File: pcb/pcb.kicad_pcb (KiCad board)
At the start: 2 copper layers, 100 x 88.7 mm, 65 parts, among them J1 AudioJack4, J2 USB_C_Receptacle_USB2.0, SW1 Switch, SW10 Switch, SW11 Switch, SW12 Switch, SW13 Switch, SW14 Switch, SW15 Switch, SW16 Switch, SW17 Switch, SW18 Switch, SW2 Switch, SW3 Switch, SW4 Switch, SW5 Switch, SW6 Switch, SW7 Switch, SW8 Switch, SW9 Switch, U1 MCU_rp2040-zero, U2 MCU_rp2040-zero, U3 RollerEncoder_EVQWGD001

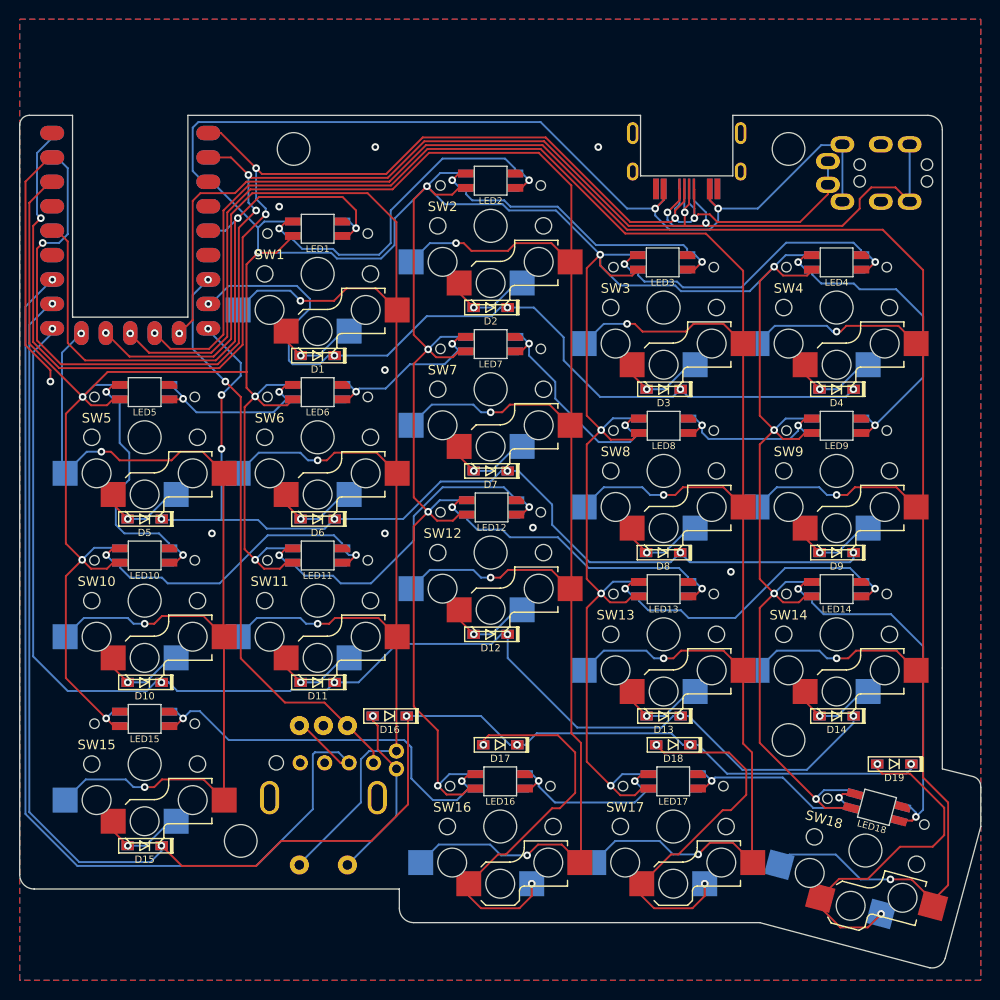
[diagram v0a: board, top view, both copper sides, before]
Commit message: small PCB updates
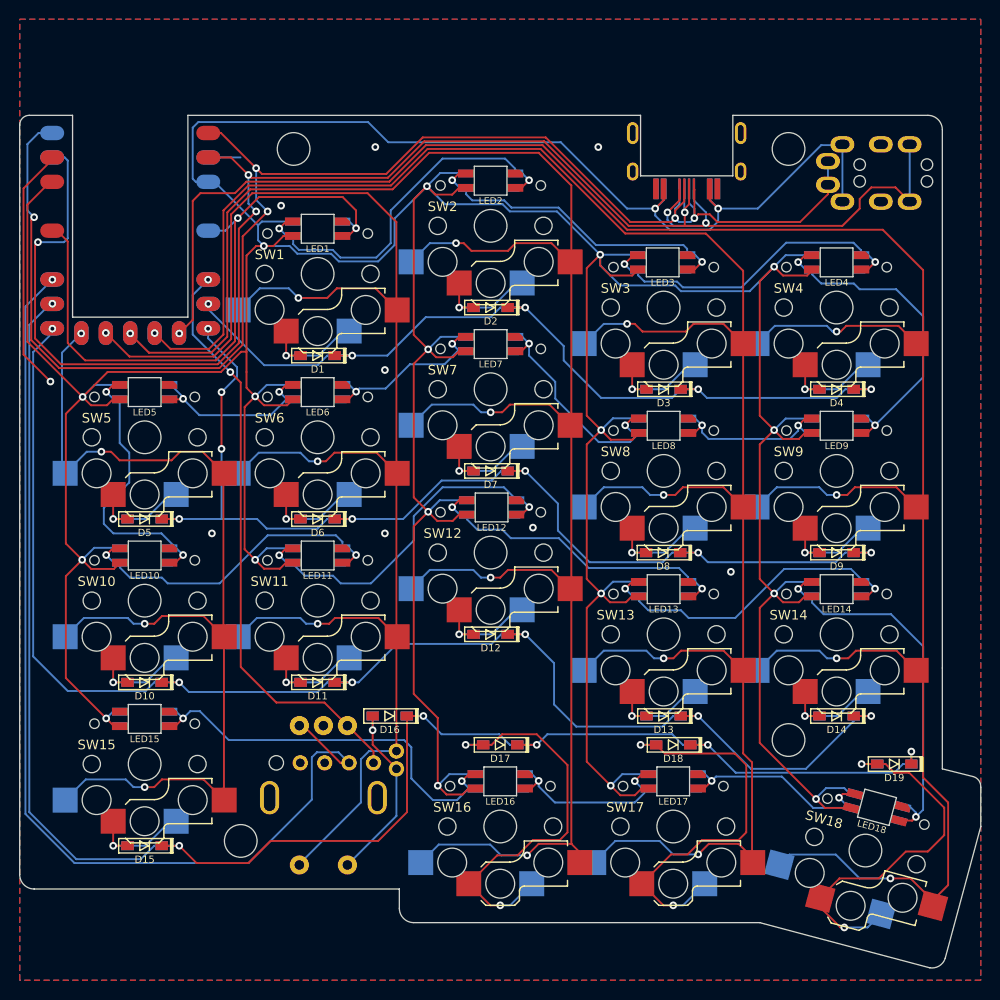
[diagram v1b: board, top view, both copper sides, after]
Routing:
- net row2: track 136.0 -> 149.7 mm
- net row1: track 103.8 -> 114.4 mm
- net row3: track 166.0 -> 175.1 mm
- net row0: track 87.3 -> 93.6 mm
- net Net-(D18-Pad2): track 37.9 -> 42.0 mm
- net GND: track 26.2 -> 29.9 mm
- net Net-(D19-Pad2): track 36.4 -> 39.3 mm
- net Net-(D14-Pad2): track 9.29 -> 11.7 mm
- net Net-(D13-Pad2): track 9.29 -> 11.7 mm
- net Net-(D4-Pad2): track 9.26 -> 11.7 mm
- net Net-(D8-Pad2): track 9.26 -> 11.7 mm
- net Net-(D9-Pad2): track 9.29 -> 11.7 mm
- net Net-(D7-Pad2): track 9.26 -> 11.7 mm
- net Net-(D6-Pad2): track 9.26 -> 11.7 mm
- net Net-(D12-Pad2): track 9.26 -> 11.7 mm
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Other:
- board text added: "github.com/zzeneg/smol"
- board text added: "smol"
- board text added: "v1.1"
